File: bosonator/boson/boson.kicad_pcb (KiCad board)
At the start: 2 copper layers, 21 x 21 mm, 8 parts, among them P1 DF40HC(4.0)-80DS-0.4V(51), P2 USB_C_Plug_USB2.0, U1 AMS1117-3.3

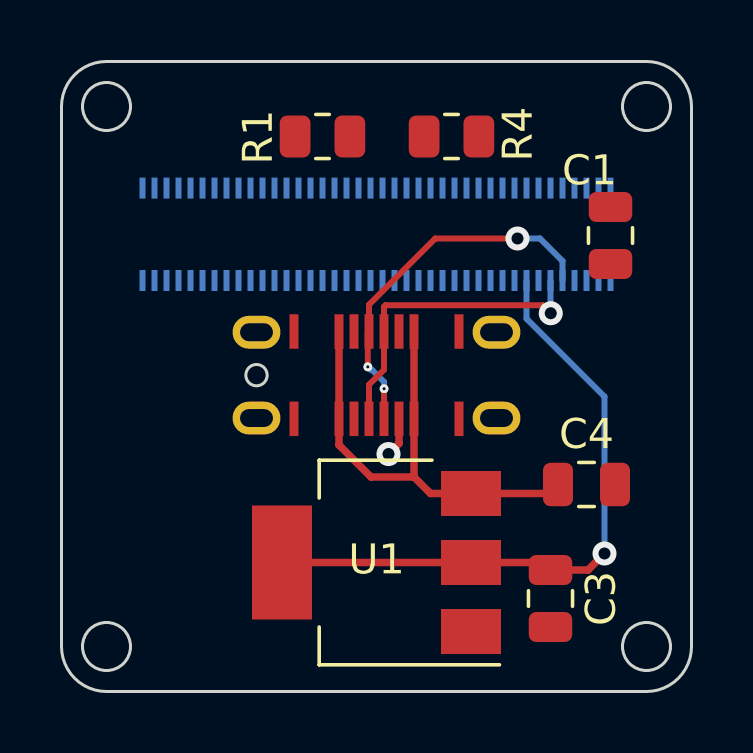
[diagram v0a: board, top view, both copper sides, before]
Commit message: [Boson] Quick & dirty routing
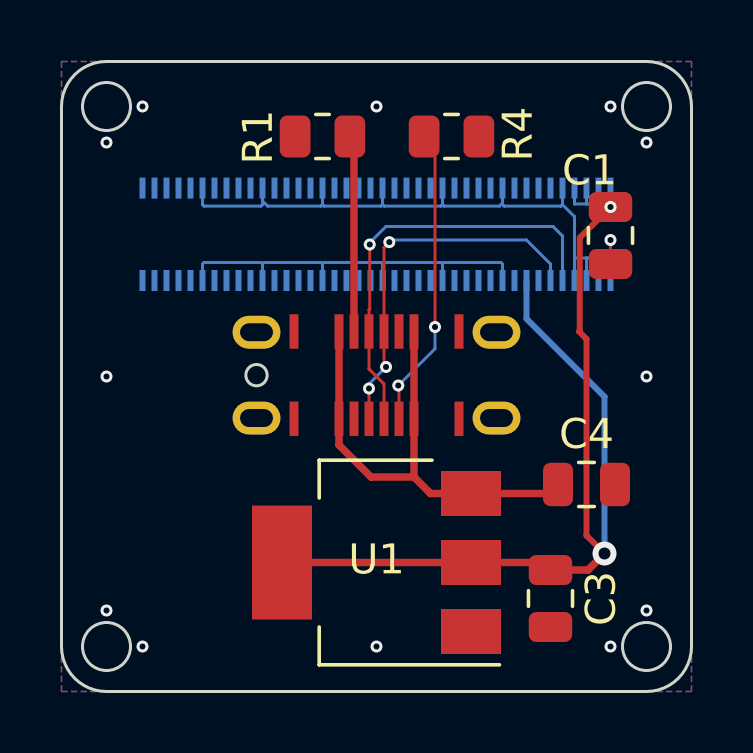
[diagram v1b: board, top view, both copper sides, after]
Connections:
- C3 pad 2: Net-(U1-GND) -> GND
- C4 pad 2: Net-(U1-GND) -> GND
- U1 pad 1: Net-(U1-GND) -> GND
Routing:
- net GND: track 0.00 -> 38.4 mm, vias 0 -> 13
- net +3.3V: track 21.3 -> 36.9 mm, vias 1 -> 2
- net Net-(P2-CC2): track 1.32 -> 10.1 mm, vias 1 -> 2
- net Net-(P2-CC1): track 0.00 -> 6.56 mm
- net /USB_D_P: track 12.4 -> 14.4 mm, vias 3 -> 1
- net /USB_D_N: track 10.7 -> 12.5 mm, vias 1 -> 3
- added copper zone on B.Cu, net GND
- added copper zone on F.Cu, net GND
